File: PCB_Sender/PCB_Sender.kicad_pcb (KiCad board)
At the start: 2 copper layers, 82.5 x 79 mm, 29 parts, among them J1 Power-Pass_MCU, J2 Header A, J3 NTC_0-3, J4 NTC_Internal, J5 Power-Pass_PSU, J7 Header B, SW1 SW_Wuerth_450301014042, U1 ESP32-DEVKITC-32D, U2 TP4056 Module, U3 DC/DC Module

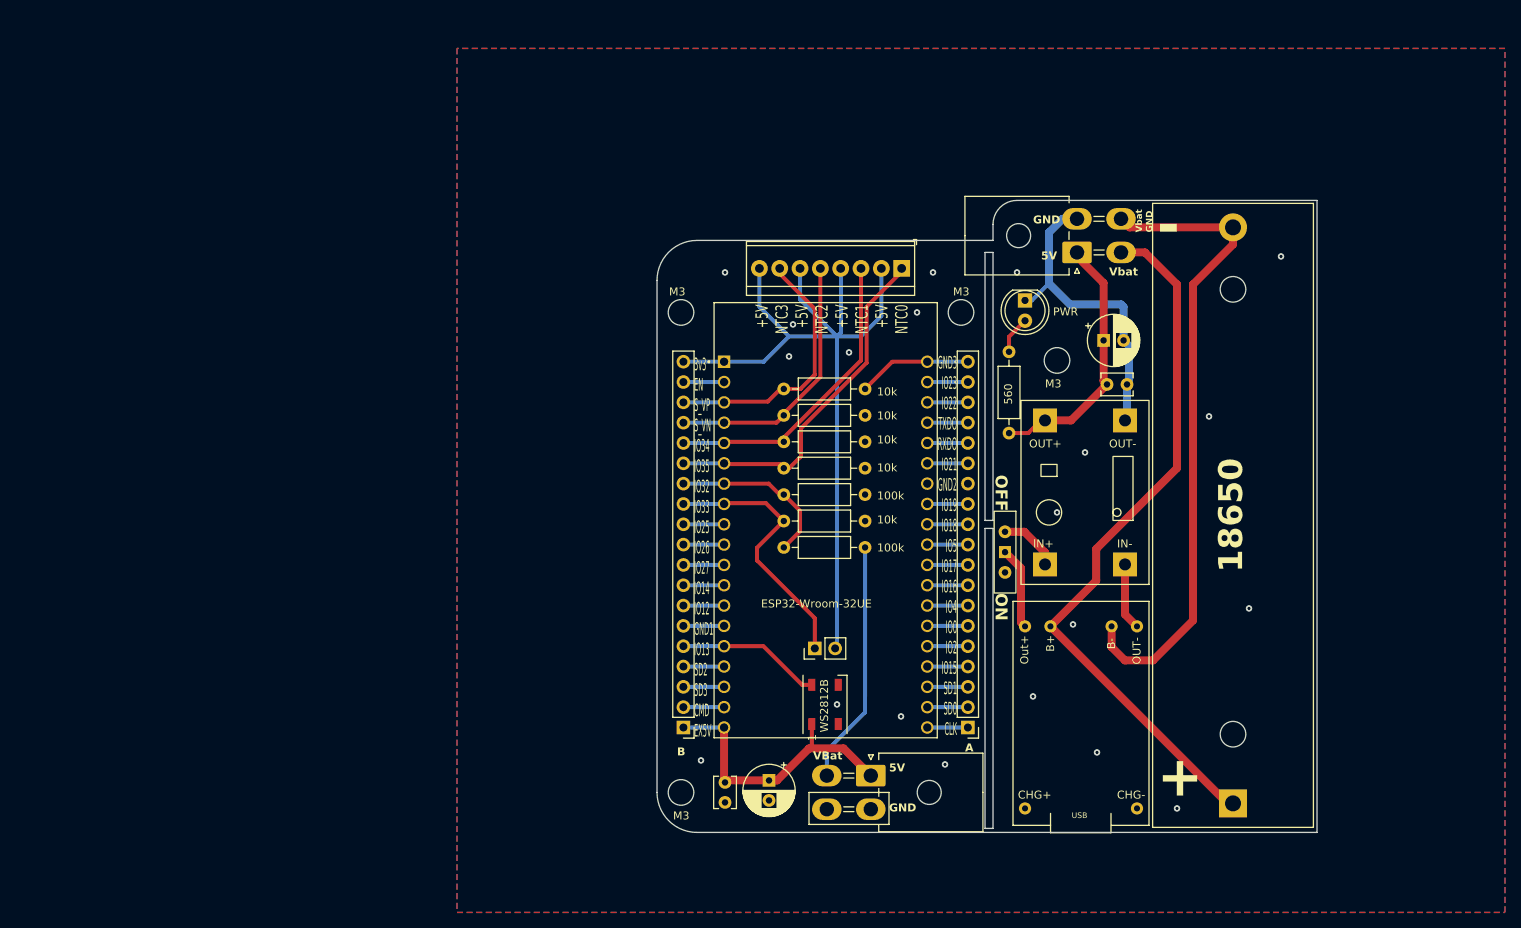
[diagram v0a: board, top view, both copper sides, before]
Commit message: WiP commit
Commited work in progress
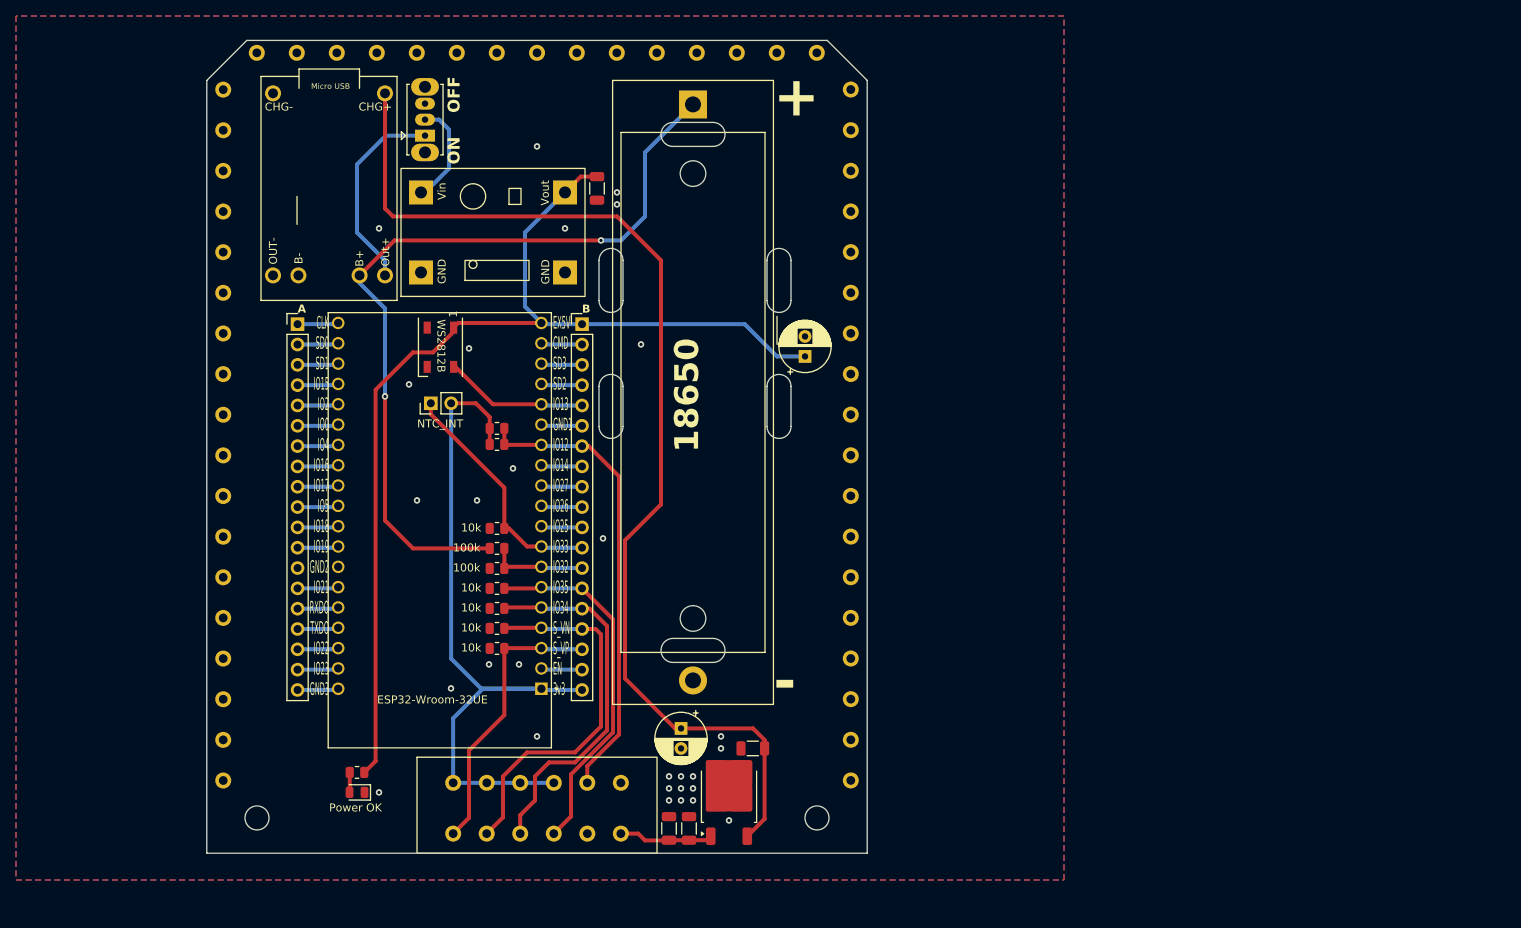
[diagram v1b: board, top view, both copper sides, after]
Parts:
- removed H1, H2, H3, H4: MountingHole, MountingHole:MountingHole_3.2mm_M3_DIN965
- removed J1: Power-Pass_MCU, Connector_Molex:Molex_Mini-Fit_Jr_5569-04A2_2x02_P4.20mm_Horizontal
- removed J3: NTC_0-3, TerminalBlock_TE-Connectivity:TerminalBlock_TE_282834-8_1x08_P2.54mm_Horizontal
- removed J5: Power-Pass_PSU, Connector_Molex:Molex_Mini-Fit_Jr_5569-04A2_2x02_P4.20mm_Horizontal
- added C5: 50V, 100nF, Capacitor_SMD:C_1206_3216Metric, F.Cu at (166.5, 138.5)
- added C6: 10V, 220uF, Capacitor_THT:CP_Radial_D6.3mm_P2.50mm, F.Cu at (168.0, 126.0)
- added G1: AUGA-Tech-LOGO, 0_user_lib:AUGA-Tech-footprint, B.Cu at (172.0, 97.5)
- added J6: DTM13-12PA, 0_user_lib:DTM13-12PA-R008, F.Cu at (150.0, 40.0)
- added R12: 100K, Resistor_SMD:R_0805_2012Metric, F.Cu at (145.0, 88.5)
- added R9: 100K, Resistor_SMD:R_0805_2012Metric, F.Cu at (145.0, 90.5)
- added U4: LM7805_TO220, Package_TO_SOT_SMD:TO-252-2, F.Cu at (174.0, 134.4)
- C1: value 10V, 220uF -> 50V, 100nF; footprint Capacitor_THT:CP_Radial_D6.3mm_P2.50mm -> Capacitor_SMD:C_1206_3216Metric
- C2, C4: value 100nF -> 50V, 100nF; footprint Capacitor_THT:C_Disc_D3.8mm_W2.6mm_P2.50mm -> Capacitor_SMD:C_1206_3216Metric
- D2: footprint LED_THT:LED_D5.0mm -> LED_SMD:LED_0805_2012Metric
- R1, R2, R3, R4, R5, R6, R7: footprint Resistor_THT:R_Axial_DIN0207_L6.3mm_D2.5mm_P10.16mm_Horizontal -> Resistor_SMD:R_0805_2012Metric
- R8: value 560 -> 680; footprint Resistor_THT:R_Axial_DIN0207_L6.3mm_D2.5mm_P10.16mm_Horizontal -> Resistor_SMD:R_0805_2012Metric
- SW1: value SW_Wuerth_450301014042 -> On-Off Switch; footprint Button_Switch_THT:SW_Slide-03_Wuerth-WS-SLTV_10x2.5x6.4_P2.54mm -> Button_Switch_THT:SW_Slide_SPDT_Straight_CK_OS102011MS2Q
- U1: footprint local_lib:MODULE_ESP32-DEVKITC-32D -> 0_user_lib:MODULE_ESP32-DEVKITC-32D
- U2: footprint local_lib:TP4056-Module -> 0_user_lib:TP4056-Module
- U3: footprint local_lib:DCDC_StepUp -> 0_user_lib:DCDC_StepUp
- moved U2 114.6 mm to (124.0, 58.5), turned to 180 degrees
- moved BT1 110.4 mm to (169.5, 48.0), turned to -90 degrees
- moved D2 103.7 mm to (127.5, 134.0), turned to 180 degrees
- moved J2 97.8 mm to (120.1, 75.5), turned to 0 degrees
- moved R8 97.0 mm to (127.5, 131.5), turned to 0 degrees
- moved SW1 89.3 mm to (136.0, 51.9), turned to 90 degrees
- moved U3 80.8 mm to (144.5, 64.0), turned to 90 degrees
- moved C4 68.3 mm to (157.5, 58.5), turned to -90 degrees
- moved D1 65.6 mm to (137.9, 78.4), turned to -90 degrees
- moved J4 56.9 mm to (136.7, 85.4)
- moved J7 52.0 mm to (155.6, 75.5), turned to 0 degrees
- moved R4 48.3 mm to (145.0, 116.0), turned to 180 degrees
- moved U1 48.3 mm to (137.8, 101.3), turned to 180 degrees
- moved R7 46.9 mm to (145.0, 106.0), turned to 0 degrees
- moved R3 44.7 mm to (145.0, 113.5), turned to 180 degrees
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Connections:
- net /IO12 renamed /Wheel_Side
- BT1 pad 1: /BAT+ -> +BATT
- BT1 pad 2: /BAT- -> GND
- C1 pad 1: +5V -> VCC
- C2 pad 1: +5V -> +5C
- C3 pad 1: /PSU_5V -> +5V
- C3 pad 2: /PSU_GND -> GND
- C4 pad 1: /PSU_5V -> +5V
- C4 pad 2: /PSU_GND -> GND
- D2 pad 1: /PSU_GND -> GND
- J7 pad 6: /GND1 -> GND
- R6 pad 2: VCC -> +BATT
- R8 pad 2: /PSU_5V -> +5V
- U1 pad J2-14: /GND1 -> GND
- U2 pad 1: unconnected-(U2-CHG+-Pad1) -> +5C
- U2 pad 2: unconnected-(U2-CHG--Pad2) -> GND
- U2 pad 4: Net-(U2-OUT-) -> GND
- U2 pad 5: /BAT+ -> +BATT
- U2 pad 6: /BAT- -> GND
- U3 pad 2: Net-(U2-OUT-) -> GND
- U3 pad 3: /PSU_5V -> +5V
- U3 pad 4: /PSU_GND -> GND
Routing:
- net +5C: track 0.00 -> 139.3 mm
- net +BATT: track 0.00 -> 101.7 mm, vias 0 -> 2
- net +5V: track 36.6 -> 132.1 mm
- net /BAT+: track 89.9 -> 0.00 mm
- net /BAT-: track 81.2 -> 0.00 mm
- net /Wheel_Side: track 5.08 -> 57.9 mm
- net /PSU_GND: track 39.7 -> 0.00 mm
- net /PSU_5V: track 32.8 -> 0.00 mm
- net VCC: track 30.5 -> 11.8 mm
- net Net-(SW1-B): track 10.3 -> 25.3 mm
- net /NTC_2: track 33.2 -> 46.7 mm
- net +3V3: track 101.3 -> 92.5 mm
- net /VBat: track 21.4 -> 12.6 mm
- net Net-(U2-OUT-): track 8.36 -> 0.00 mm
- net /NTC_1: track 38.3 -> 46.1 mm
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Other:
- board size 82.5 x 79 mm -> 82.6 x 101.6 mm
- board text added: "3v3"
- board text added: "CLK SD0 SD1 IO15 IO2 IO0 IO4 IO16 IO17 IO5 IO18 IO19 GND2 IO21 RXDO TXDO IO22 IO23 GND3"
- board text added: "D.Vaitiekus 2024-05-22 OTA-Sender-MCU Rev C AUGA Tech"
- board text added: "EX5V CMD SD3 SD2 IO13 GND1 IO12 IO14 IO27 IO26 IO25 IO33 IO32 IO35 IO34 S_VN S_VP EN 3v3"
- board text added: "NTC0"
- board text added: "NTC1"
- board text added: "NTC2"
- board text added: "NTC3"
- board text added: "NTC_INT"
- board text added: "Power OK"
- board text added: "Vcc"
- board text added: "WS"
- board text removed: "+5V NTC3 +5V NTC2 +5V NTC1 +5V NTC0"
- board text removed: "3v3 EN S_VP S_VN IO34 IO35 IO32 IO33 IO25 IO26 IO27 IO14 IO12 GND1 IO13 SD2 SD3 CMD EX5V"
- board text removed: "560"
- board text removed: "5V"
- board text removed: "D.Vaitiekus 2024-05-03 OTA-Sender-MCU Rev B AUGA Tech"
- board text removed: "D.Vaitiekus 2024-05-03 OTA-Sender-PSU Rev B AUGA Tech"
- board text removed: "GND3 IO23 IO22 TXDO RXDO IO21 GND2 IO19 IO18 IO5 IO17 IO16 IO4 IO0 IO2 IO15 SD1 SD0 CLK"
- board text removed: "IN+"
- board text removed: "IN-"
- board text removed: "M3"
- board text removed: "OUT+"
- board text removed: "OUT-"
- board text removed: "PWR"
- board text removed: "VBat"
- board text removed: "Vbat"
- board text removed: "Vbat GND"
